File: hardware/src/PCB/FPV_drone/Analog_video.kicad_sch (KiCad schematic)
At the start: 1 part, among them IC7 AT7456E

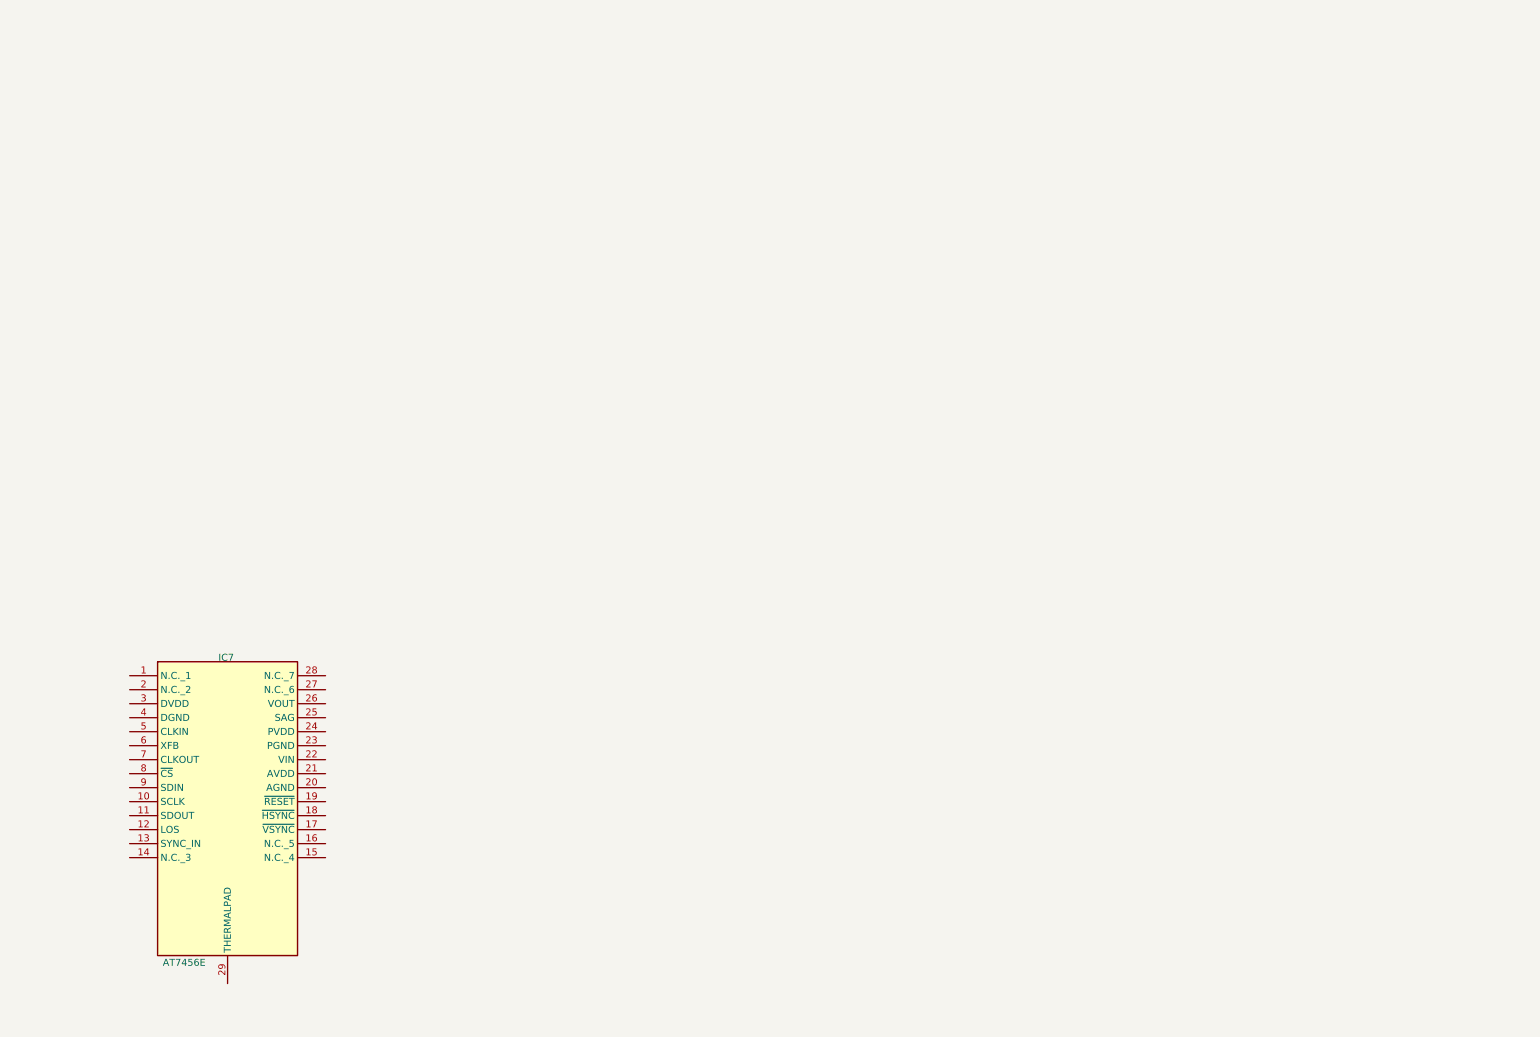
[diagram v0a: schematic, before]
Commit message: Update: schem almost finish
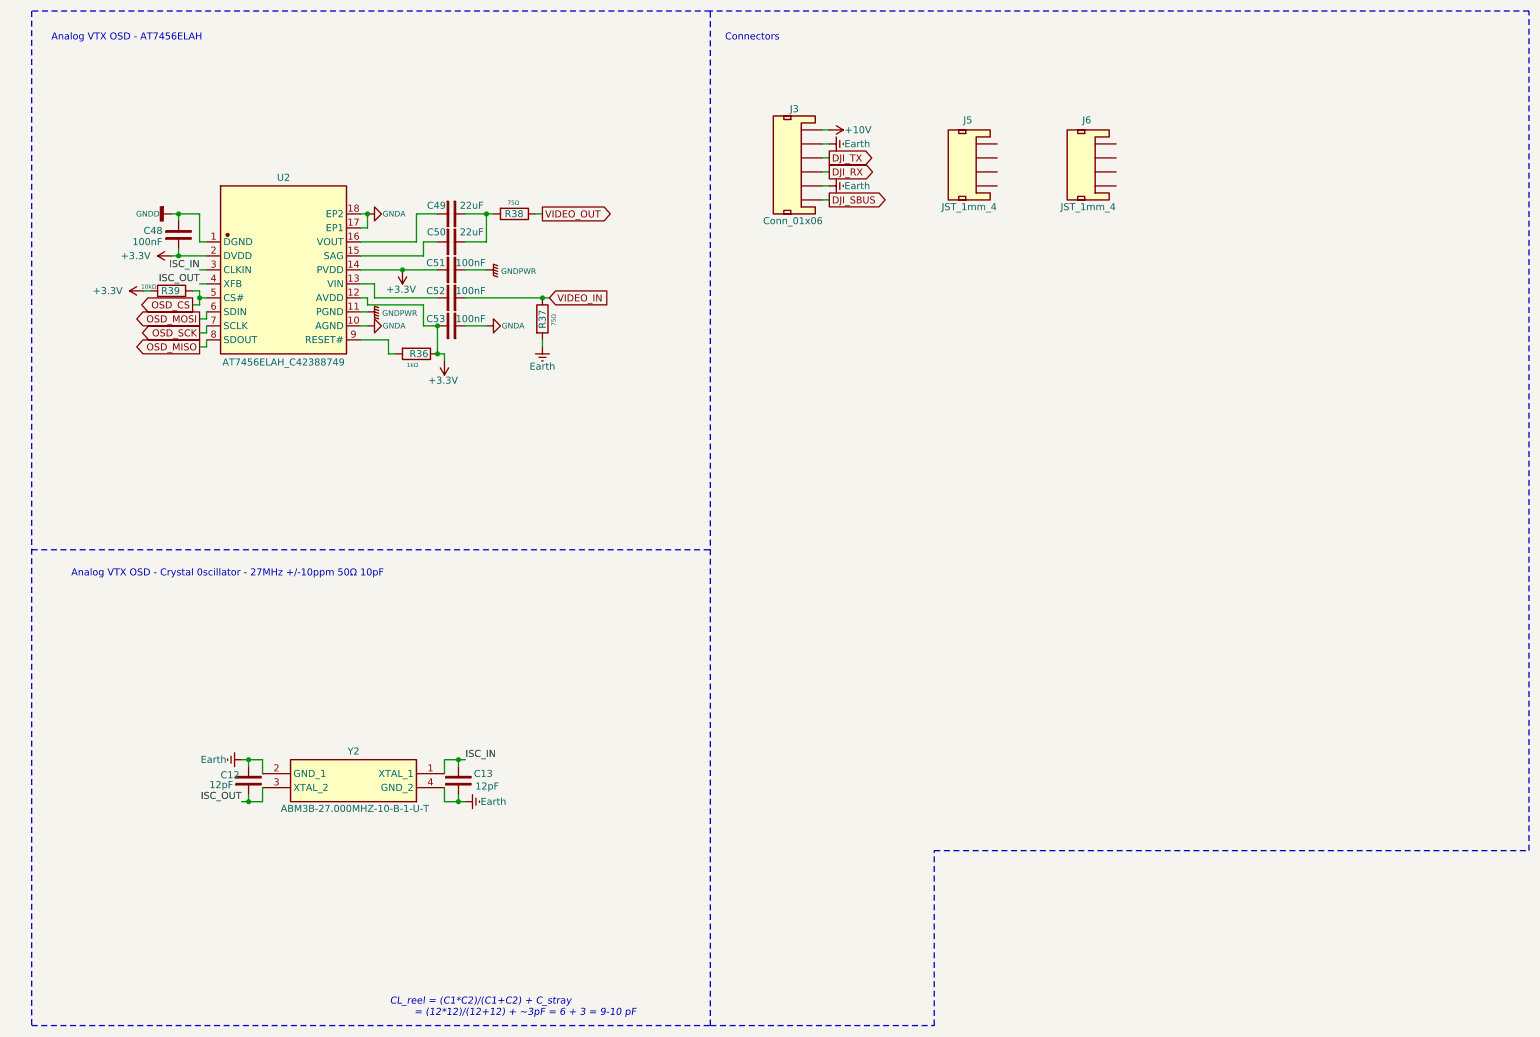
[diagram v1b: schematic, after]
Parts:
- removed IC7: AT7456E, SOP65P640X120-29N, symbol lib:AT7456E
- added C12, C13: 12pF, Capacitor_THT:C_Disc_D3.0mm_W2.0mm_P2.50mm, symbol PCM_SL_Devices:Capacitor_NP
- added C48, C51, C52, C53: 100nF, Capacitor_THT:C_Disc_D3.0mm_W2.0mm_P2.50mm, symbol PCM_SL_Devices:Capacitor_NP
- added C49, C50: 22uF, Capacitor_THT:C_Disc_D3.0mm_W2.0mm_P2.50mm, symbol PCM_SL_Devices:Capacitor_NP
- added J3: Conn_01x06, PCM_SparkFun-Connector:JST_1x06_P1.0mm_Horizontal_SMD, symbol PCM_SparkFun-Connector:Conn_01x06_JST_P1.0mm_Horizontal_SMD
- added J5, J6: JST_1mm_4, PCM_SparkFun-Connector:JST_1x04_P1.0mm_Horizontal_SMD, symbol PCM_SparkFun-Connector:Conn_01x04_JST_P1.0mm_Horizontal_SMD
- added R36: 1kΩ, symbol Device:R
- added R37, R38: 75Ω, symbol Device:R
- added R39: 10kΩ, symbol Device:R
- added U2: AT7456ELAH_C42388749, symbol lib:AT7456ELAH_C42388749
- added Y2: ABM3B-27.000MHZ-10-B-1-U-T, ABM3B, symbol lib:ABM3B-8.000MHZ-10-D1G-T
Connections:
- new net: C49.1, U2.16 (VOUT)
- new net: C49.2, C50.2, R38.2
- new net: C52.2, U2.13 (VIN)
- new net: R36.2, U2.9 (RESET#)
- new net: C50.1, U2.15 (SAG)
- new net +10V: J3.6
- new net +3.3V: C48.1, C51.2, C53.2, R36.1, R39.1, U2.12 (AVDD), U2.14 (PVDD), U2.2 (DVDD)
- new net DJI_RX: J3.3
- new net DJI_SBUS: J3.1
- new net DJI_TX: J3.4
- new net Earth: C12.2, C13.1, J3.2, J3.5, R37.2, Y2.2 (GND_1), Y2.4 (GND_2)
- new net GNDA: C53.1, U2.10 (AGND), U2.17 (EP1), U2.18 (EP2)
- new net GNDD: C48.2, U2.1 (DGND)
- new net GNDPWR: C51.1, U2.11 (PGND)
- new net ISC_IN: C13.2, U2.3 (CLKIN), Y2.1 (XTAL_1)
- new net ISC_OUT: C12.1, U2.4 (XFB), Y2.3 (XTAL_2)
- new net OSD_CS: R39.2, U2.5 (CS#)
- new net OSD_MISO: U2.8 (SDOUT)
- new net OSD_MOSI: U2.6 (SDIN)
- new net OSD_SCK: U2.7 (SCLK)
- new net VIDEO_IN: C52.1, R37.1
- new net VIDEO_OUT: R38.1
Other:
- note added: "Analog VTX OSD - AT7456ELAH"
- note added: "Analog VTX OSD - Crystal 0scillator - 27MHz +/-10ppm 50Ω 10pF"
- note added: "CL_reel = (C1*C2)/(C1+C2) + C_stray = (12*12)/(12+12) + ~3pF = 6 + 3 = 9-10 pF"
- note added: "Connectors"
